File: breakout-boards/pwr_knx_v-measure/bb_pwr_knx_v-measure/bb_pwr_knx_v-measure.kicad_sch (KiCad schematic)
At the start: 50 parts, among them IC100 TPS560430, T1 BC856, T2 FZT753, T3 BC847

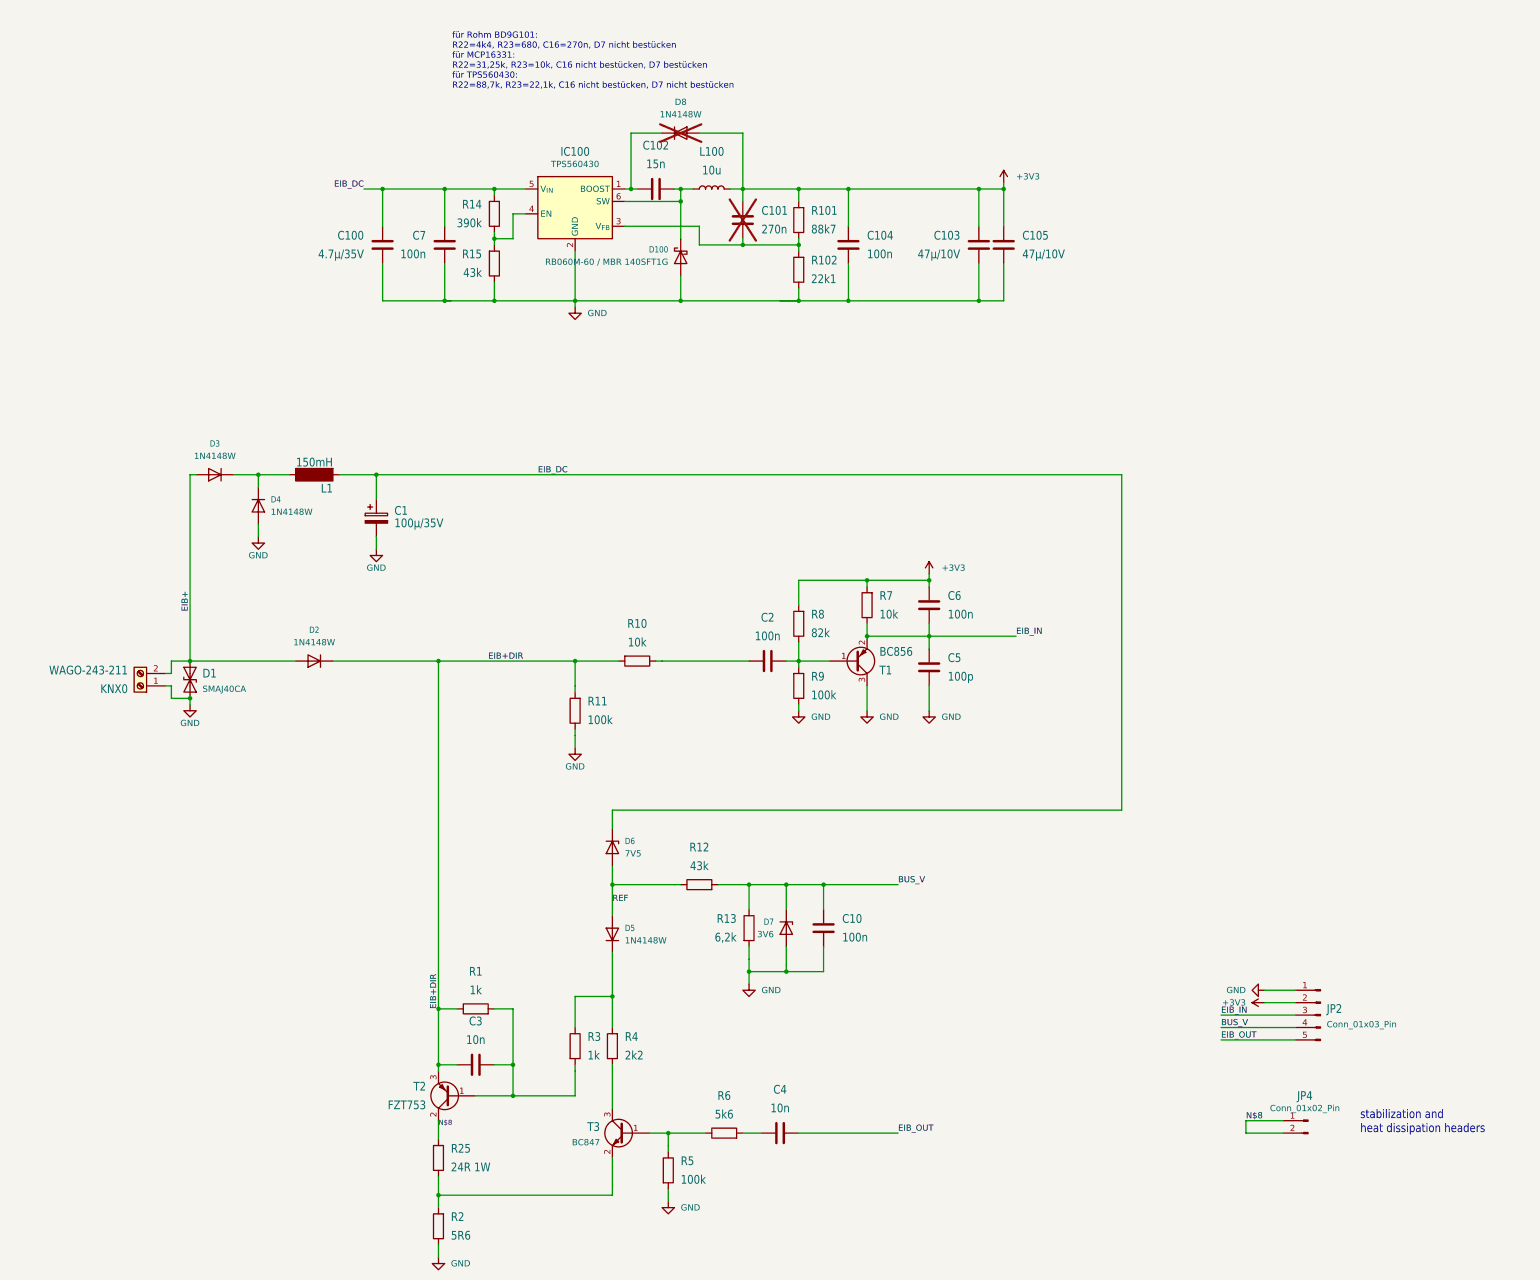
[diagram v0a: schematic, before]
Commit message: bb_pwr_knx_v-measure final
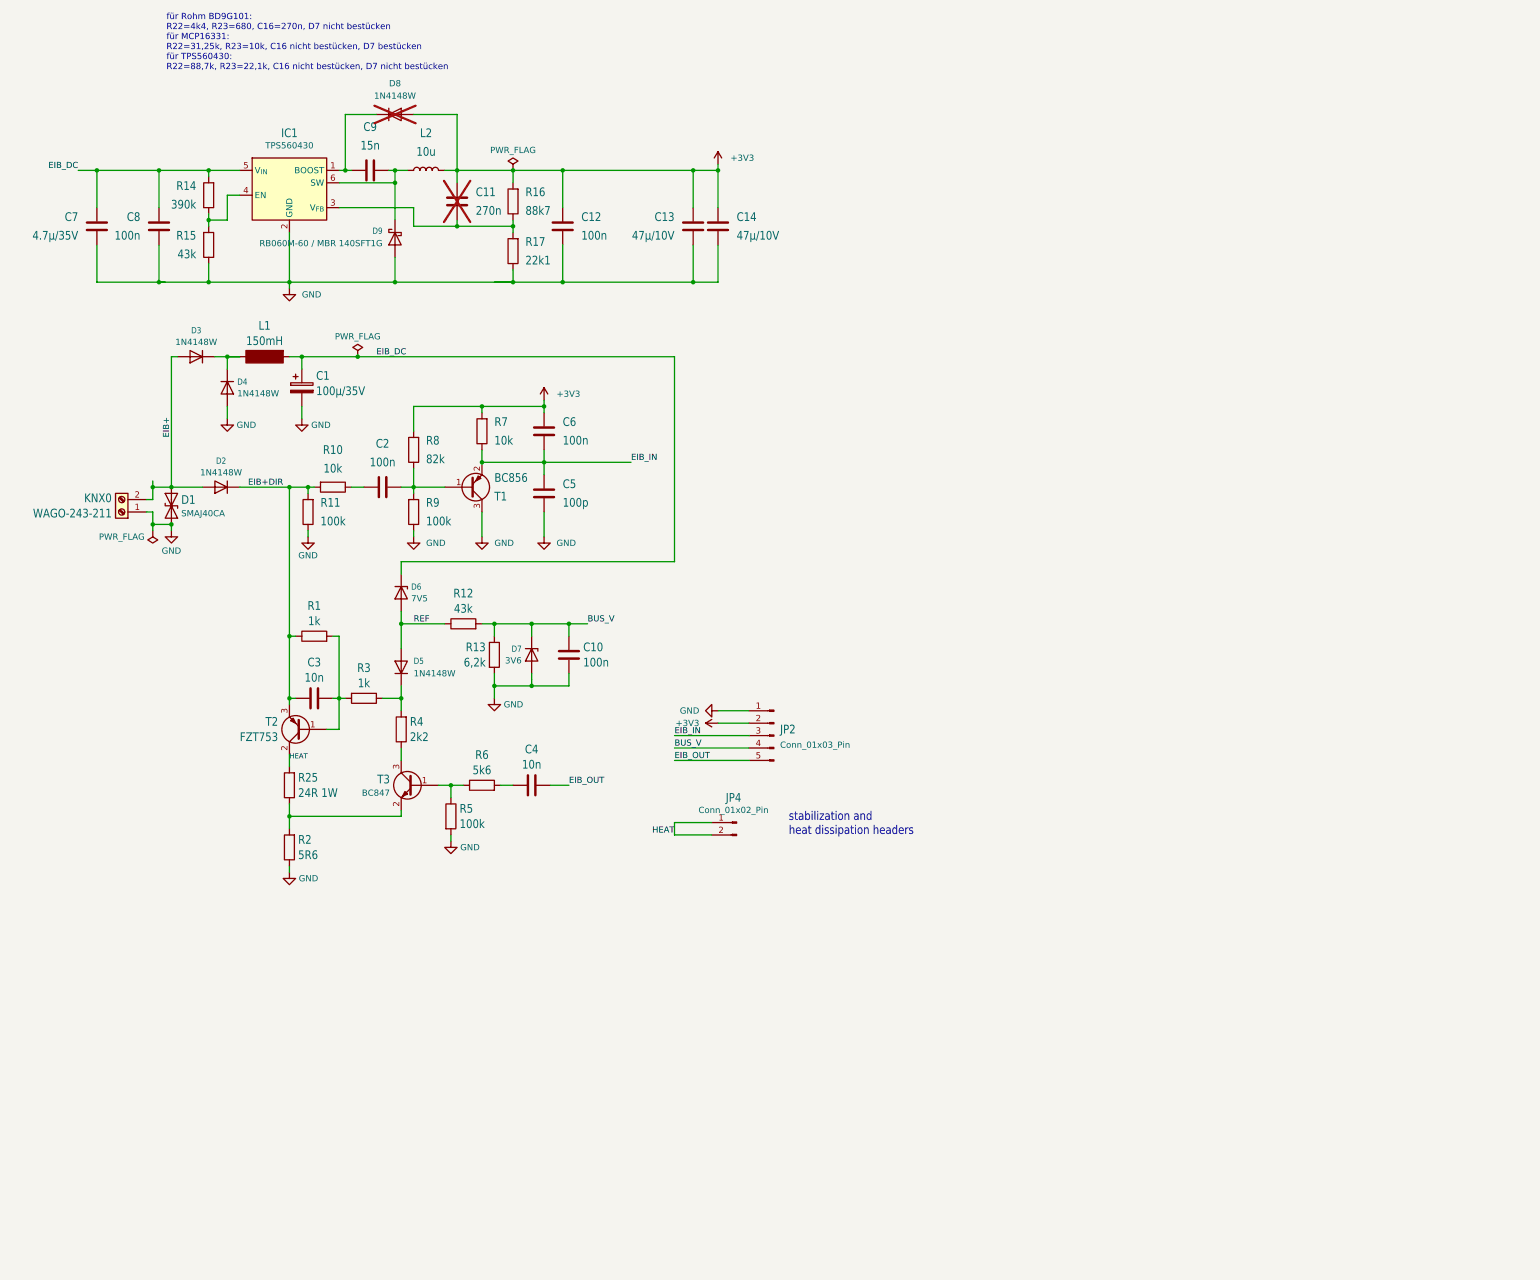
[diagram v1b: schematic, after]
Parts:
- renumbered C101 to C11, C104 to C12, C103 to C13, C105 to C14, C100 to C7, C7 to C8, C102 to C9, D100 to D9, IC100 to IC1, L100 to L2, R101 to R16, R102 to R17
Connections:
- net N$8 renamed HEAT
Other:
- moved on the sheet: C1, C10, C11, C12, C13, C14, C2, C3, C4, C5, C6, C7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
